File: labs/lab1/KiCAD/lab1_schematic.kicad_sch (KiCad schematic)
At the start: 15 parts, among them SW1 Push Button, U1 74HC595, U2 ATmega328P µC

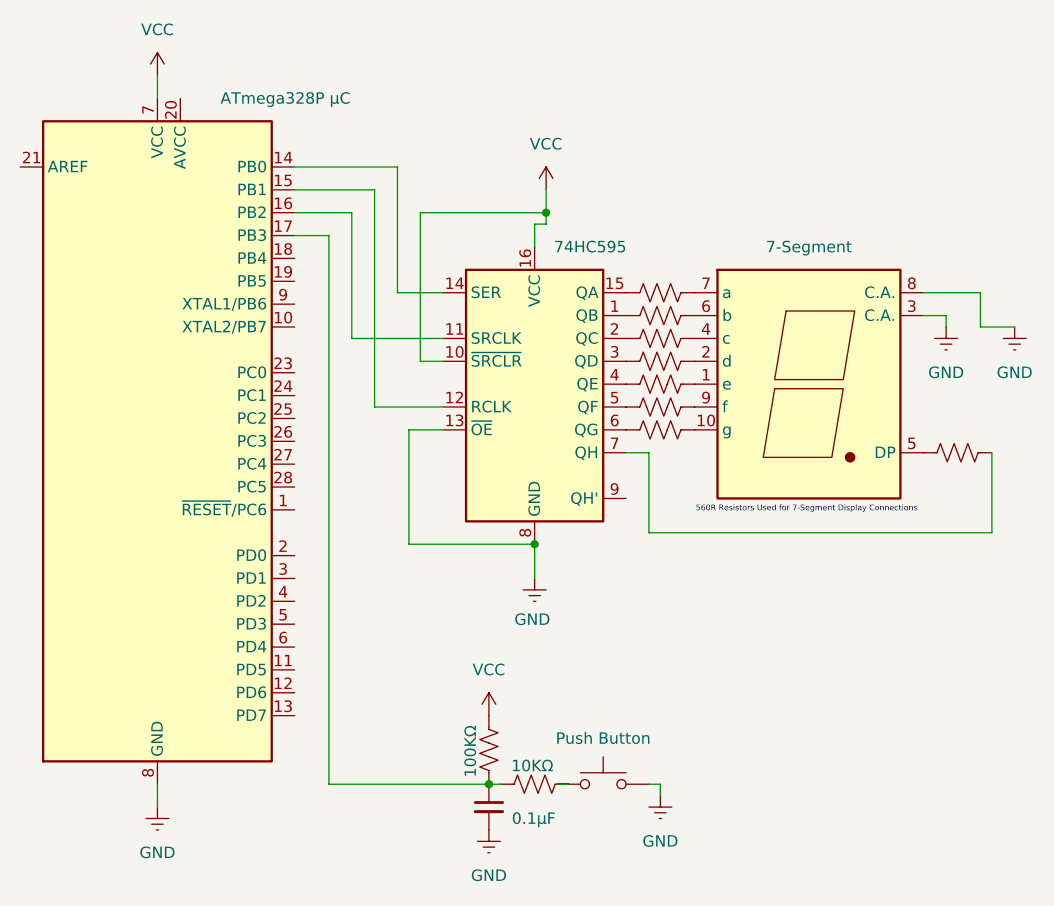
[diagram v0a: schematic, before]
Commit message: kicad
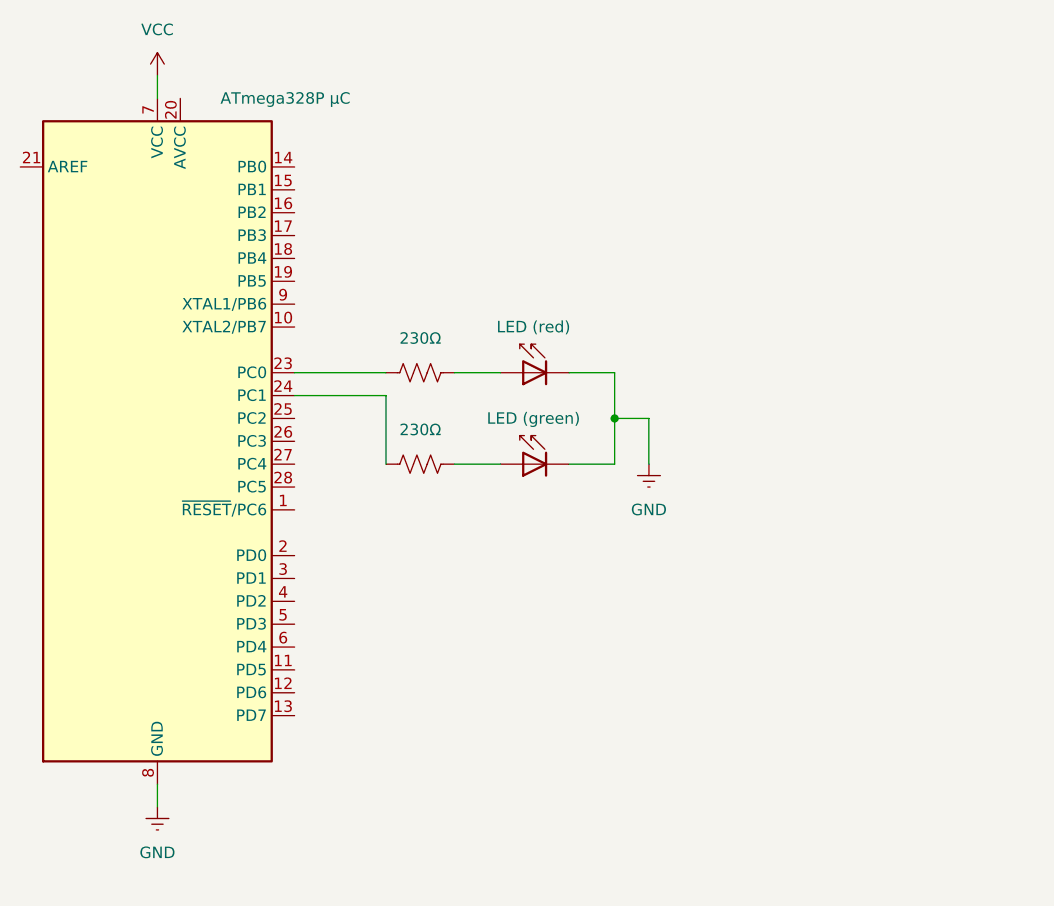
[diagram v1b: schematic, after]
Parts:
- removed AFF1: 7-Segment, Display_7Segment:7SegmentLED_LTS6760_LTS6780, symbol Display_Character:LTS-6960HR
- removed C1: 0.1µF, symbol Device:C_Small
- removed R10, R3, R4, R5, R6, R7, R8, R9: 10K, symbol Device:R_US
- removed SW1: Push Button, symbol Switch:SW_Push
- removed U1: 74HC595, symbol 74xx:74HC595
- added D1: LED (red), LED_THT:LED_D5.0mm_IRGrey, symbol LED:LD274
- added D2: LED (green), LED_THT:LED_D5.0mm_IRGrey, symbol LED:LD274
- R1: value 10KΩ -> 230Ω
- R2: value 100KΩ -> 230Ω
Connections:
- net GND: now also D1.1 (K), D2.1 (K)
- net VCC: no longer R2.1
- net at R1.1: now also U2.23 (PC0)
- net at U2.24 (PC1): now also R2.1
- new net: D1.2 (A), R1.2
- new net: D2.2 (A), R2.2
- now unconnected: U2.17 (PB3)
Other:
- note removed: "560R Resistors Used for 7-Segment Display Connections"
- title: 7-Segment Display Controlled by Push Button -> Blinky
